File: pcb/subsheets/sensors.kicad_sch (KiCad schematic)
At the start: 5 parts, among them U2 KP212K1409XTMA1, U3 AT30TS75A-SS8M

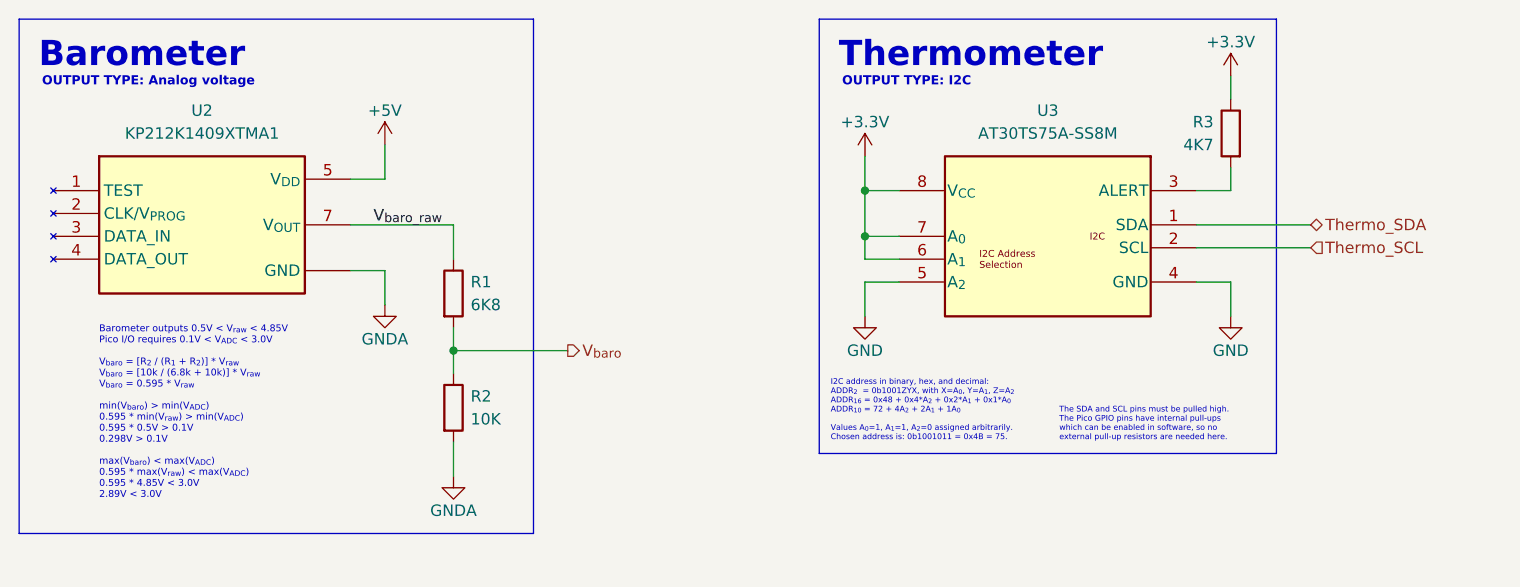
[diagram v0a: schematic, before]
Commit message: mostly finished schematic
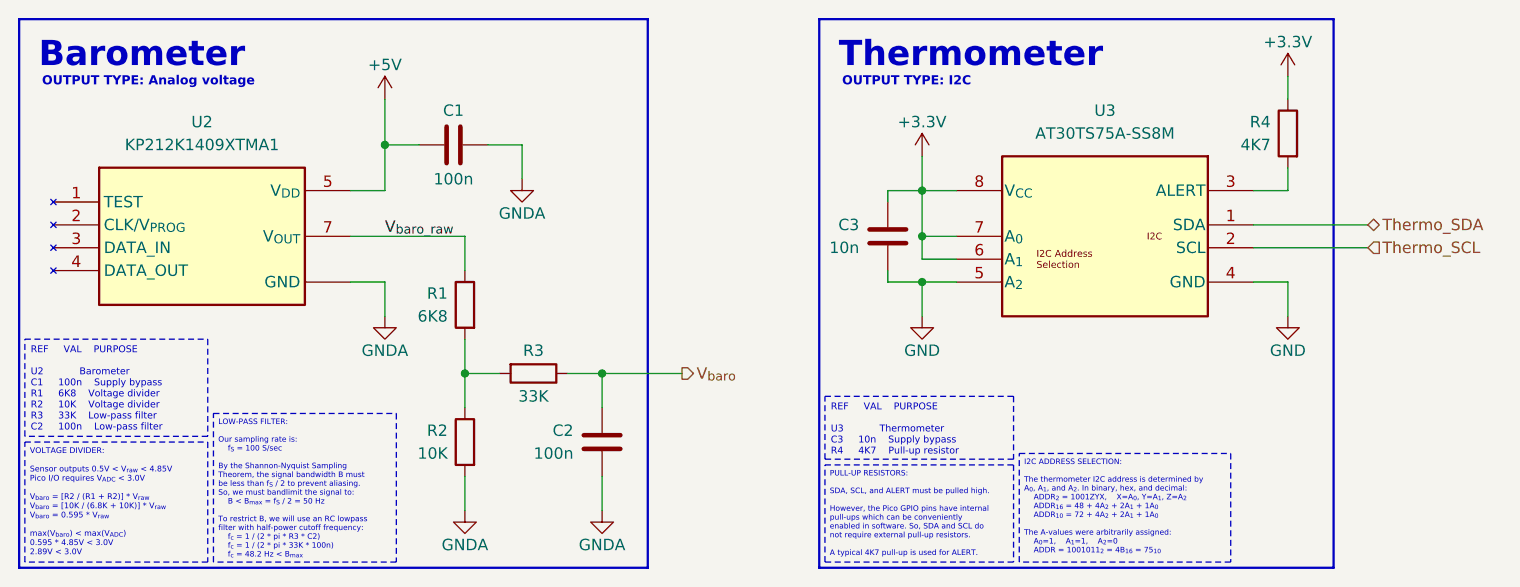
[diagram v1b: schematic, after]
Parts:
- added C1, C2: 100n, symbol Device:C
- added C3: 10n, symbol Device:C
- added R3: 33K, symbol Device:R
- renumbered R3 to R4
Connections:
- net +3.3V: now also C3.2
- net +5V: now also C1.1
- net GND: now also C3.1
- net GNDA: now also C1.2, C2.2
- net V_{baro}: now also C2.1, R3.1; no longer R1.2, R2.1
- new net: R1.2, R2.1, R3.2
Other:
- note removed: "Barometer outputs 0.5V < V_{raw} < 4.85V Pico I/O requires 0.1V < V_{ADC} < 3.0V V_{baro} = [R_{2} / (R_{1} + R_{2})] * V_{raw} V_{baro} = [10k / (6.8k + 10k)] * V_{raw} V_{baro} = 0.595 * V_{raw} min(V_{baro}) > min(V_{ADC}) 0.595 * min(V_{raw}) > min(V_{ADC}) 0.595 * 0.5V > 0.1V 0.298V > 0.1V max(V_{baro}) < max(V_{ADC}) 0.595 * max(V_{raw}) < max(V_{ADC}) 0.595 * 4.85V < 3.0V 2.89V < 3.0V"
- note removed: "I2C address in binary, hex, and decimal: ADDR_{2} = 0b1001ZYX, with X=A_{0}, Y=A_{1}, Z=A_{2} ADDR_{16} = 0x48 + 0x4*A_{2} + 0x2*A_{1} + 0x1*A_{0} ADDR_{10} = 72 + 4A_{2} + 2A_{1} + 1A_{0} Values A_{0}=1, A_{1}=1, A_{2}=0 assigned arbitrarily. Chosen address is: 0b1001011 = 0x4B = 75."
- note removed: "The SDA and SCL pins must be pulled high. The Pico GPIO pins have internal pull-ups which can be enabled in software, so no external pull-up resistors are needed here."
- moved on the sheet: R1, R2, R4, U2, U3
